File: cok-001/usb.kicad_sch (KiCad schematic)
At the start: 51 parts, among them J3301 USB_A_Stacked, J3302 USB_A_Stacked, U3302 BU9869W, Y3301 12MHz

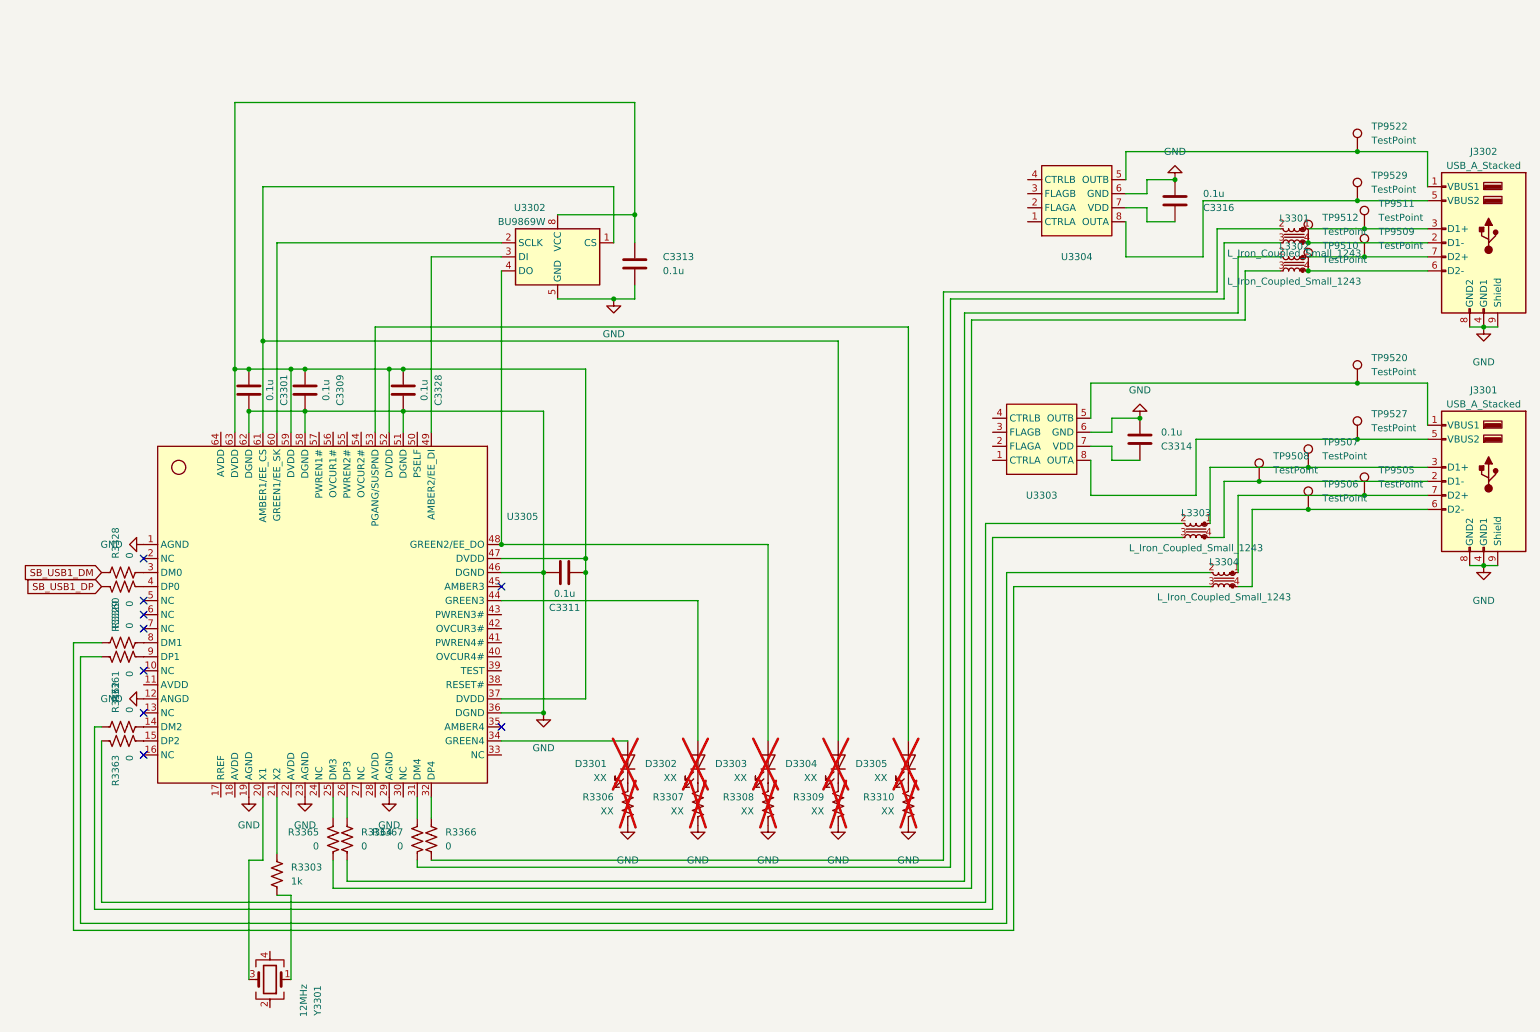
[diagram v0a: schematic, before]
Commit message: rdy
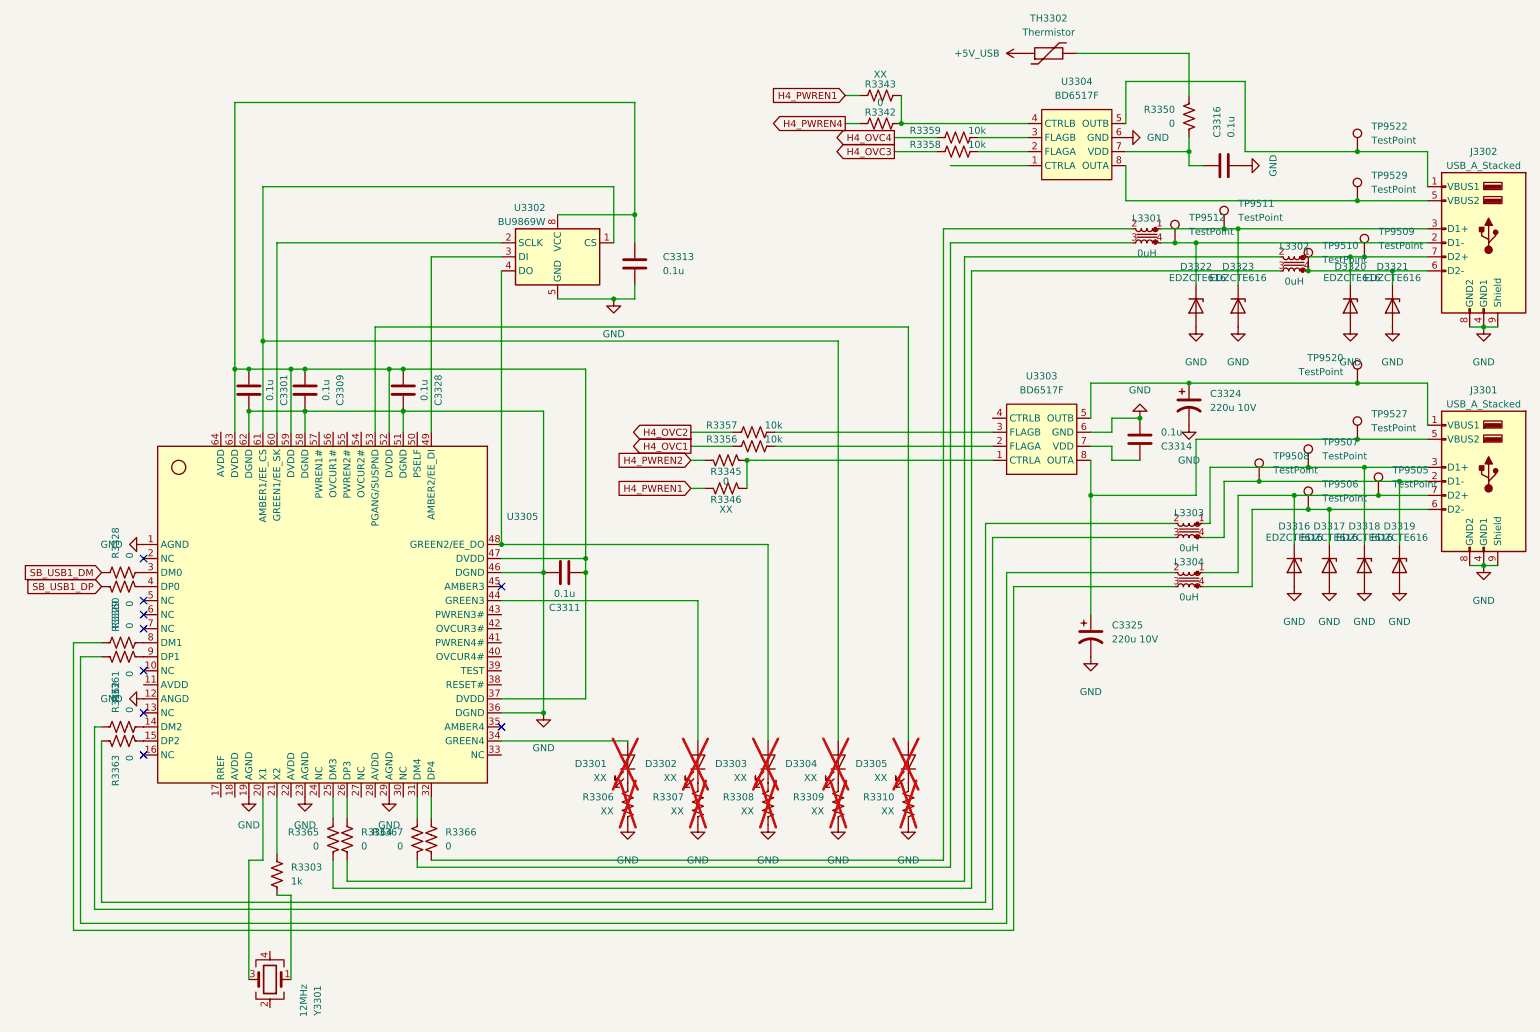
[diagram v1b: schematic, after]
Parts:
- added C3324, C3325: 220u 10V, Capacitor_Tantalum_SMD:CP_EIA-6032-28_Kemet-C, symbol Device:C_Polarized_US
- added D3316, D3317, D3318, D3319, D3320, D3321, D3322, D3323: EDZCTE616, Diode_SMD:D_SOD-923, symbol Device:D_Zener
- added R3342, R3345: 0, Resistor_SMD:R_0402_1005Metric, symbol Device:R_US
- added R3343, R3346: XX, Resistor_SMD:R_0402_1005Metric, symbol Device:R_US
- added R3350: 0, Resistor_SMD:R_0603_1608Metric, symbol Device:R_US
- added R3356, R3357, R3358, R3359: 10k, Resistor_SMD:R_0402_1005Metric, symbol Device:R_US
- added TH3302: Thermistor, symbol Device:Thermistor
- L3301, L3302, L3303, L3304: value L_Iron_Coupled_Small_1243 -> 0uH
- U3303, U3304: value ~ -> BD6517F
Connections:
- net GND: now also C3324.2, C3325.2, D3316.2 (A), D3317.2 (A), D3318.2 (A), D3319.2 (A), D3320.2 (A), D3321.2 (A), D3322.2 (A), D3323.2 (A)
- net at J3302.2 (D1-), L3301.4, TP9512.1: now also D3322.1 (K)
- net at J3302.3 (D1+), L3301.1, TP9511.1: now also D3323.1 (K)
- net at J3302.6 (D2-), L3302.4, TP9510.1: now also D3321.1 (K)
- net at J3302.7 (D2+), L3302.1, TP9509.1: now also D3320.1 (K)
- net at J3301.1 (VBUS1), TP9520.1, U3303.5 (OUTB): now also C3324.1
- net at J3301.2 (D1-), L3303.4, TP9508.1: now also D3319.1 (K)
- net at J3301.3 (D1+), L3303.1, TP9507.1: now also D3318.1 (K)
- net at J3301.5 (VBUS2), TP9527.1, U3303.8 (OUTA): now also C3325.1
- net at J3301.6 (D2-), L3304.4, TP9506.1: now also D3317.1 (K)
- net at J3301.7 (D2+), L3304.1, TP9505.1: now also D3316.1 (K)
- net at U3304.2 (FLAGA): now also R3358.2
- net at U3304.3 (FLAGB): now also R3359.2
- net at U3304.4 (CTRLB): now also R3342.2, R3343.2
- net at C3316.1, U3304.7 (VDD): now also R3350.1
- net at U3303.1 (CTRLA): now also R3345.2, R3346.2
- net at U3303.2 (FLAGA): now also R3356.2
- net at U3303.3 (FLAGB): now also R3357.2
- new net: R3350.2, TH3302.2
- new net +5V_USB: TH3302.1
- new net H4_OVC1: R3356.1
- new net H4_OVC2: R3357.1
- new net H4_OVC3: R3358.1
- new net H4_OVC4: R3359.1
- new net H4_PWREN1: R3343.1, R3346.1
- new net H4_PWREN2: R3345.1
- new net H4_PWREN4: R3342.1
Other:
- moved on the sheet: C3316, L3301, L3303, L3304, TP9505, TP9511, TP9512, U3304
